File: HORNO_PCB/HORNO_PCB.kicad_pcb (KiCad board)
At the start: 2 copper layers, 407.9 x 406.6 mm, 104 parts, among them J0_1 Terminales de tornillo espaci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, J0_10 Terminales de tornillo espaci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, J0_11 Terminales de tornillo espaci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, J0_12 Terminales de tornillo espaci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, J0_13 Terminales de tornillo espaci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, J0_14 Terminales de tornillo espaci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, J0_15 Terminales de tornillo espaci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, J0_18 Terminales de tornillo espaci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, J0_2 Terminales de tornillo espaci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, J0_3 Terminales de tornillo espaci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, J0_4 Terminales de tornillo espaci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, J0_5 Terminales de tornillo espaci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, J0_6 Terminales de tornillo espaci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, J0_7 Terminales de tornillo espaci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, J0_8 Terminales de tornillo espaci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, J0_9 Terminales de tornillo espaci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, J1 switch, J10 switch, J11 switch, J12 switch, J13 switch, J14 switch, J15 switch, J16 switch, J17 switch, J18 switch, J19 switch, J20 switch, J21 switch, J22 switch, J23 switch, J24 Screw_Terminal_01x20, J25 Screw_Terminal_01x20, J26 Screw_Terminal_01x20, J27 Screw_Terminal_01x20, J7 24VDC, J8 switch, J9 switch, K1 Relay 1, K2 Relay 2, K6 Relay 4, K7 Relay 3, K8 Relay 2, K9 Relay 1, Q1 2N2222, Q2 2N2222, Q6 IRG4PF50W, Q7 IRG4PF50W, U1 TLP521-1, U10 LM741, U15 TLP250, U17 LM741, U18 LM741, U19 TLP250, U2 TLP521-1, U25 UDN2981A, U3 TLP521-1, U4 TLP521-1, U9 LM741

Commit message: Tamaño de PCB  y ruteo
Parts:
- J0_1: value Terminales de tornillo espaciados en 5mm -> Alimentacion dispositivo serial
- J1: value switch -> +5V +24V
- moved F1 178.5 mm to (363.5, 313.9), turned to 90 degrees
- moved J7 151.9 mm to (332.4, 307.3), turned to 90 degrees
- moved J0_1 112.5 mm to (375.7, 177.6), turned to 180 degrees
- moved R23 93.5 mm to (461.3, 367.1)
- moved J1 84.4 mm to (370.4, 187.0)
- moved J0_10 84.4 mm to (486.7, 182.1)
- moved J0_13 83.1 mm to (486.7, 356.9)
- moved C9 82.1 mm to (454.3, 370.9)
- moved J0_3 81.6 mm to (355.5, 177.6), turned to 180 degrees
- moved R21 79.3 mm to (461.3, 339.3)
- moved J16 77.8 mm to (311.9, 375.5)
- moved J17 77.8 mm to (332.9, 375.5)
- moved J8 77.8 mm to (332.9, 332.3)
- moved J9 77.8 mm to (311.9, 332.3)
- moved U18 76.2 mm to (465.1, 375.1)
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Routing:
- net Net-(J0_13-Pin_2): track 0.00 -> 877.8 mm, vias 0 -> 3
- net Net-(D10-A): track 0.00 -> 568.1 mm, vias 0 -> 1
- net Net-(J8-Pin_1): track 0.00 -> 360.1 mm, vias 0 -> 2
- net Net-(J11-Pin_1): track 0.00 -> 264.2 mm, vias 0 -> 1
- net Net-(J14-Pin_1): track 0.00 -> 247.8 mm, vias 0 -> 3
- net Net-(J25-Pin_8): track 0.00 -> 184.6 mm, vias 0 -> 1
- net Net-(J25-Pin_9): track 0.00 -> 160.4 mm, vias 0 -> 1
- net Net-(J13-Pin_1): track 0.00 -> 113.5 mm, vias 0 -> 1
- net Net-(J25-Pin_10): track 0.00 -> 112.3 mm, vias 0 -> 1
- net Net-(J24-Pin_18): track 0.00 -> 97.8 mm, vias 0 -> 1
- net Net-(J24-Pin_4): track 0.00 -> 96.8 mm
- net Net-(J24-Pin_17): track 0.00 -> 88.5 mm, vias 0 -> 1
- net Net-(J24-Pin_10): track 0.00 -> 80.2 mm
- net Net-(J25-Pin_11): track 0.00 -> 76.5 mm, vias 0 -> 1
- net Net-(D14-K): track 0.00 -> 75.9 mm
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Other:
- board size 407.9 x 406.6 mm -> 198 x 218 mm

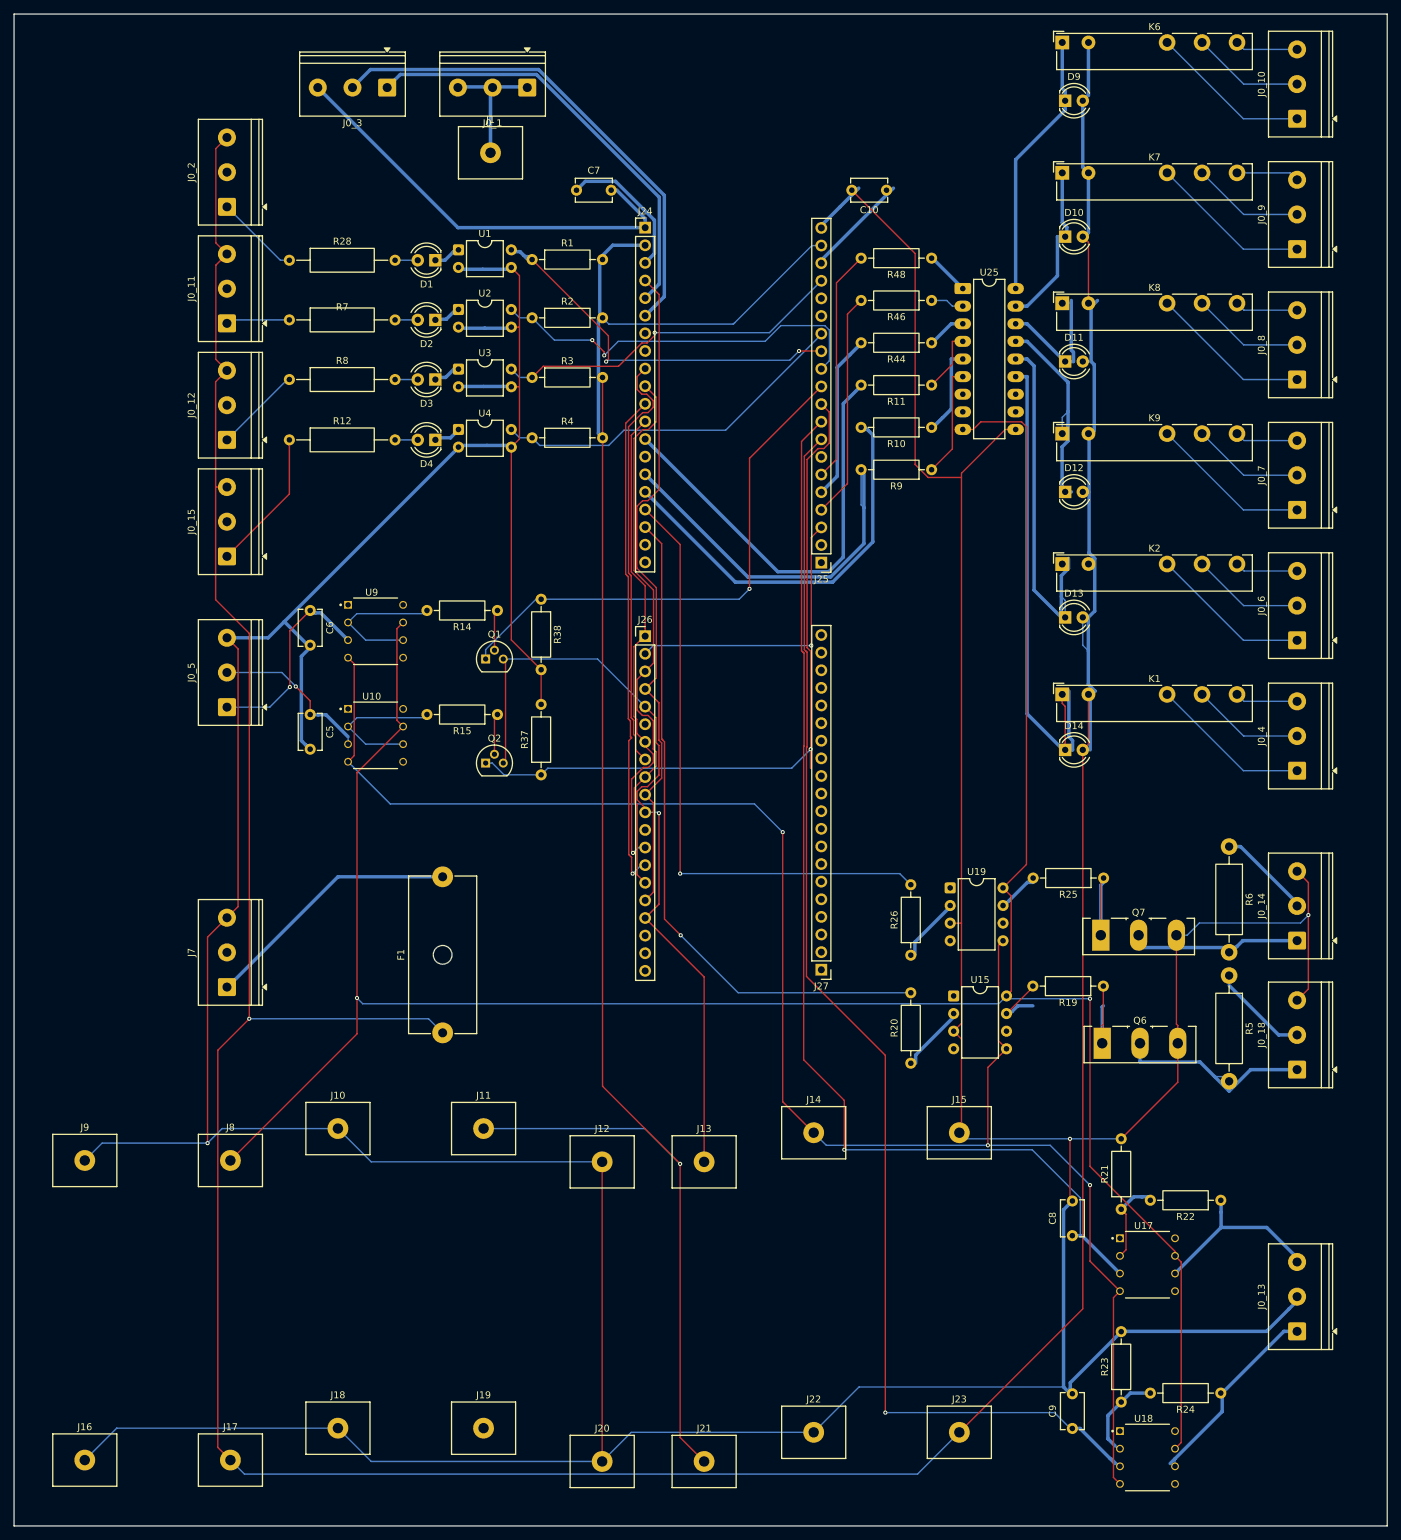
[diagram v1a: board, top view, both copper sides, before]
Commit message: Check point 1
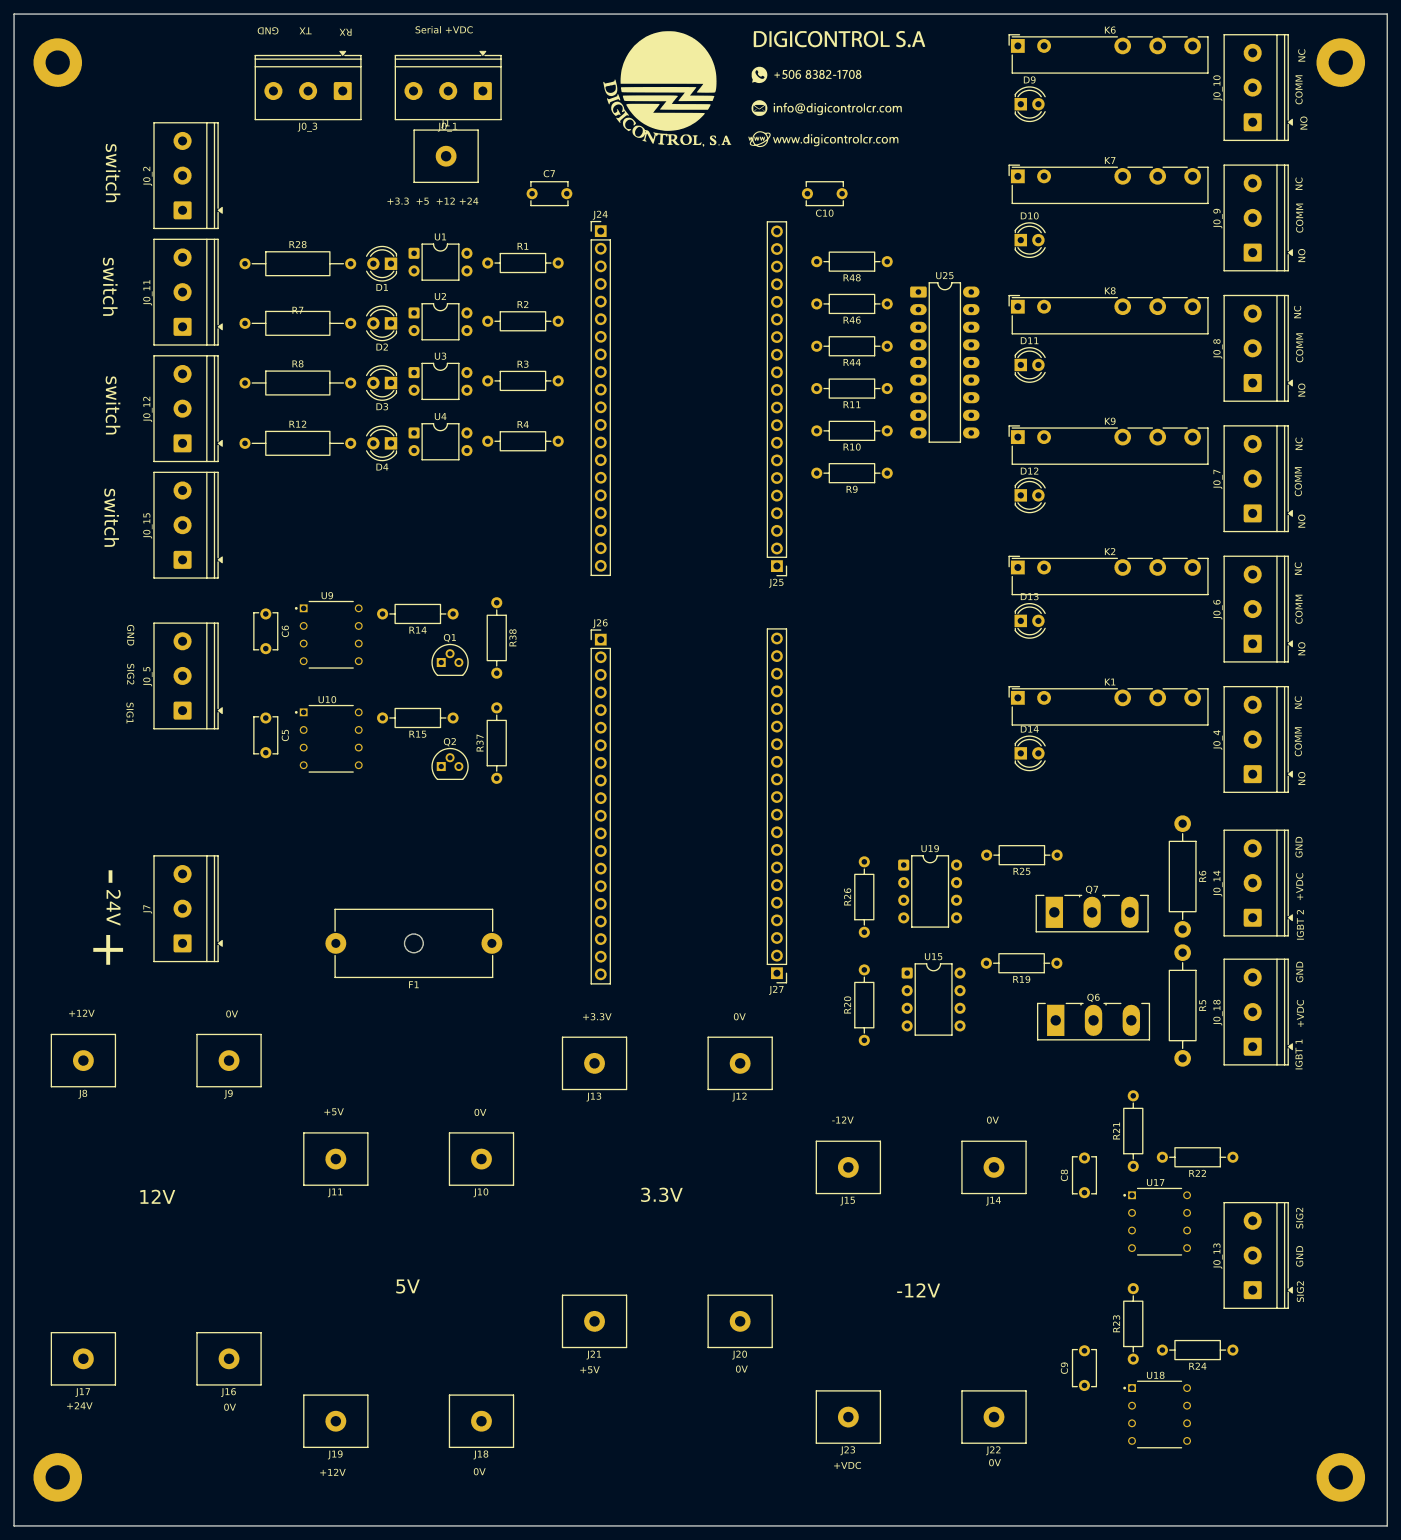
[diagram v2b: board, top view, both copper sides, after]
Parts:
- added G***: LOGO, images:Info DGC, F.Cu at (409.6, 177.6)
- added REF**: MountingHole_3.5mm_Pad, MountingHole:MountingHole_3.5mm_Pad, F.Cu at (493.0, 378.0)
- added REF**: MountingHole_3.5mm_Pad, MountingHole:MountingHole_3.5mm_Pad, F.Cu at (308.0, 174.0)
- added REF**: MountingHole_3.5mm_Pad, MountingHole:MountingHole_3.5mm_Pad, F.Cu at (308.0, 378.0)
- added REF**: MountingHole_3.5mm_Pad, MountingHole:MountingHole_3.5mm_Pad, F.Cu at (493.0, 174.0)
- moved J20 28.4 mm to (406.4, 355.5), turned to 180 degrees
- moved J14 26.5 mm to (443.0, 333.3), turned to 180 degrees
- moved J22 26.1 mm to (443.0, 369.3), turned to 180 degrees
- moved J17 25.7 mm to (311.7, 360.9), turned to 180 degrees
- moved J21 25.6 mm to (385.4, 355.5), turned to 180 degrees
- moved J8 25.6 mm to (311.7, 317.9), turned to 180 degrees
- moved J16 25.4 mm to (332.7, 360.9), turned to 180 degrees
- moved J9 25.3 mm to (332.7, 317.9), turned to 180 degrees
- moved J12 24.4 mm to (406.4, 318.3), turned to 180 degrees
- moved J11 21.7 mm to (348.1, 332.1), turned to 180 degrees
- moved J19 21.3 mm to (348.1, 369.9), turned to 180 degrees
- moved J13 21.2 mm to (385.4, 318.3), turned to 180 degrees
- moved J10 21.2 mm to (369.1, 332.1), turned to 180 degrees
- moved J18 20.7 mm to (369.1, 369.9), turned to 180 degrees
- moved J15 16.8 mm to (422.0, 333.3), turned to 180 degrees
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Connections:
- J0_5 pad 3: Net-(J0_13-Pin_2) -> unconnected-(J0_5-Pin_3-Pad3)
- J14 pad 1: Net-(J14-Pin_1) -> Net-(J0_13-Pin_2)
- J15 pad 1: Net-(J0_13-Pin_2) -> Net-(J15-Pin_1)
- J19 pad 1: unconnected-(J19-Pin_1-Pad1) -> Net-(D10-A)
- J21 pad 1: Net-(J11-Pin_1) -> Net-(D10-A)
- J22 pad 1: Net-(J0_13-Pin_2) -> unconnected-(J22-Pin_1-Pad1)
- J23 pad 1: Net-(D10-A) -> unconnected-(J23-Pin_1-Pad1)
- R1 pad 2: Net-(J11-Pin_1) -> Net-(J13-Pin_1)
- R2 pad 2: Net-(J11-Pin_1) -> Net-(J13-Pin_1)
- R3 pad 2: Net-(J11-Pin_1) -> Net-(J13-Pin_1)
- R4 pad 2: Net-(J11-Pin_1) -> Net-(J13-Pin_1)
- U10 pad 4: Net-(J14-Pin_1) -> Net-(J15-Pin_1)
- U15 pad 5: Net-(J14-Pin_1) -> Net-(J15-Pin_1)
- U17 pad 4: Net-(J14-Pin_1) -> Net-(J15-Pin_1)
- U18 pad 4: Net-(J14-Pin_1) -> Net-(J15-Pin_1)
- U19 pad 5: Net-(J14-Pin_1) -> Net-(J15-Pin_1)
- U9 pad 4: Net-(J14-Pin_1) -> Net-(J15-Pin_1)
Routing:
- net Net-(J0_13-Pin_2): track 877.8 -> 0.00 mm, vias 3 -> 0
- net Net-(D10-A): track 568.1 -> 0.00 mm, vias 1 -> 0
- net Net-(J8-Pin_1): track 360.1 -> 0.00 mm, vias 2 -> 0
- net Net-(J11-Pin_1): track 264.2 -> 0.00 mm, vias 1 -> 0
- net Net-(J14-Pin_1): track 247.8 -> 0.00 mm, vias 3 -> 0
- net Net-(J25-Pin_8): track 184.6 -> 0.00 mm, vias 1 -> 0
- net Net-(J25-Pin_9): track 160.4 -> 0.00 mm, vias 1 -> 0
- net Net-(J13-Pin_1): track 113.5 -> 0.00 mm, vias 1 -> 0
- net Net-(J25-Pin_10): track 112.3 -> 0.00 mm, vias 1 -> 0
- net Net-(J24-Pin_18): track 97.8 -> 0.00 mm, vias 1 -> 0
- net Net-(J24-Pin_4): track 96.8 -> 0.00 mm
- net Net-(J24-Pin_17): track 88.5 -> 0.00 mm, vias 1 -> 0
- net Net-(J24-Pin_10): track 80.2 -> 0.00 mm
- net Net-(J25-Pin_11): track 76.5 -> 0.00 mm, vias 1 -> 0
- net Net-(D14-K): track 75.9 -> 0.00 mm
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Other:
- board text added: "+"
- board text added: "+12V"
- board text added: "+24V"
- board text added: "+3.3 +5 +12 +24"
- board text added: "+3.3V"
- board text added: "+5V"
- board text added: "+VDC"
- board text added: "-"
- board text added: "-12V"
- board text added: "0V"
- board text added: "12V"
- board text added: "24V"
- board text added: "3.3V"
- board text added: "5V"
- board text added: "COMM"
- board text added: "GND"
- board text added: "IGBT 1"
- board text added: "IGBT 2"
- board text added: "NC"
- board text added: "NO"
- board text added: "RX"
- board text added: "SIG1"
- board text added: "SIG2"
- board text added: "Serial +VDC"
- board text added: "TX"
- board text added: "switch"
